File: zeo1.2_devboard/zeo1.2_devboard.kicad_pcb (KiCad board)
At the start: 4 copper layers, 25.4 x 25.4 mm, 96 parts, among them J1 USB_C_Receptacle_USB2.0_14P, J2 JST-PH Battery, J4 Micro_SD, Q2 BC817, Q3 BC817, SW1 Boot, SW2 RESET, U1 AP2112K-3.3, U10 ESP32-S3, U11 LSM6DS3, U12 BMM150, U13 W3011, U2 MCP73871, U3 BME280, U5 USBLC6-2SC6, U6 CP2102N-QFN24, U7 W25Q128JVSIQ, U8 ANT3216LL00R2400A, U9 MAX-M10S-00B, Y1 40MHz

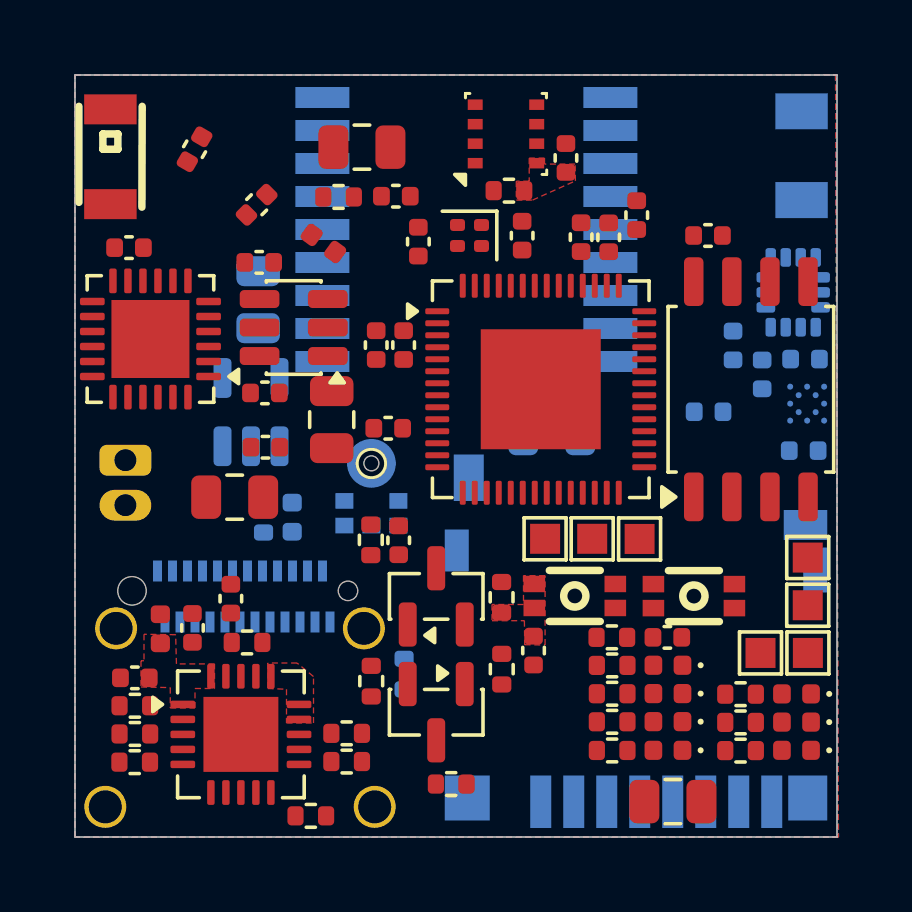
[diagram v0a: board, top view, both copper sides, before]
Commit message: new boards
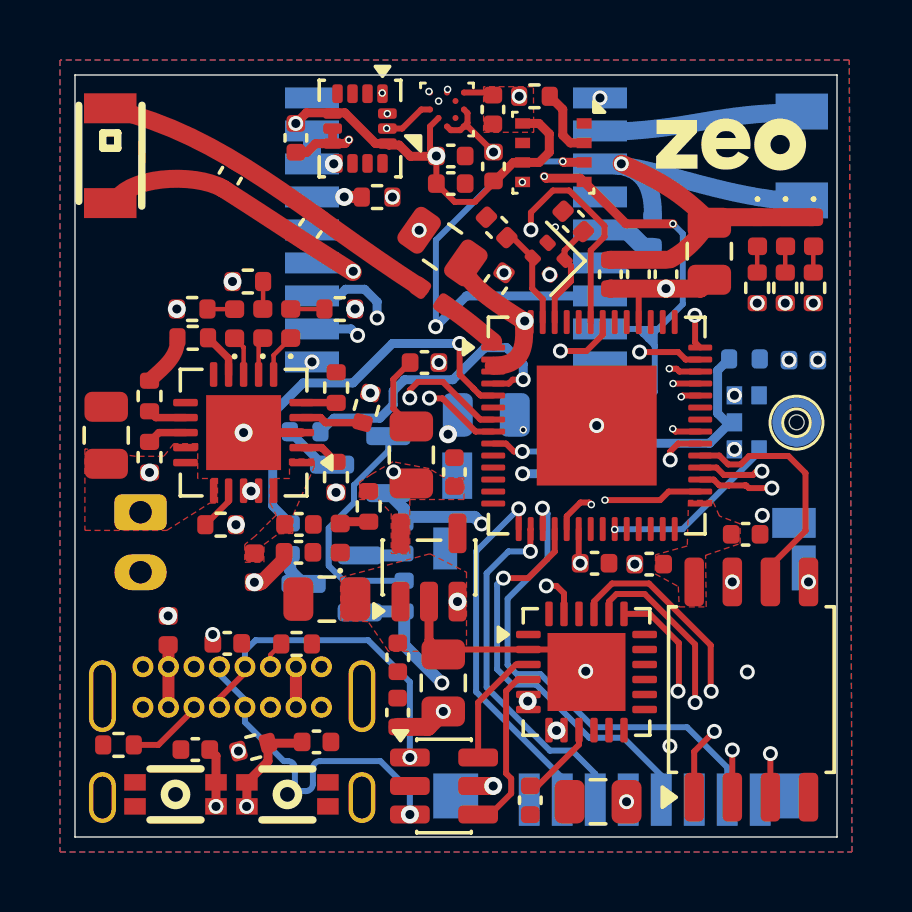
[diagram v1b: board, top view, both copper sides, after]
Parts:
- removed TP2, TP3, TP4, TP6, TP7, TP8, TP9: TestPoint, TestPoint:TestPoint_Pad_1.0x1.0mm
- added C11: 4.7uF, Capacitor_SMD:C_0805_2012Metric, F.Cu at (138.3, 99.3)
- added C12: 4.7uF, Capacitor_SMD:C_0805_2012Metric, B.Cu at (151.0, 98.6)
- added G***: LOGO, LOGO, F.Cu at (159.2, 89.6)
- C10, C38, Q2, Q3, R16, R22, R23, R24, R25: moved to B.Cu
- C19, C21, C26, C32, C33, C34, C9, F1, R1, R2, U1, U11, U12: moved to F.Cu
- J1: footprint Connector_USB:USB_C_Receptacle_Amphenol_12401610E4-2A_CircularHoles -> Connector_USB:USB_C_Receptacle_GCT_USB4085
- J2: footprint Connector_JST:JST_ZH_B2B-ZR_1x02_P1.50mm_Vertical -> Connector_JST:JST_PH_B2B-PH-K_1x02_P2.00mm_Vertical
- moved C17 22.8 mm to (152.5, 111.5), turned to 90 degrees
- moved R13 19.0 mm to (143.1, 94.2)
- moved D3 19.0 mm to (142.6, 95.6), turned to 90 degrees
- moved D2 19.0 mm to (144.5, 95.6), turned to 90 degrees
- moved R12 19.0 mm to (141.2, 95.1)
- moved D4 18.9 mm to (143.6, 95.6), turned to 90 degrees
- moved U6 18.3 mm to (154.3, 107.2), turned to 0 degrees
- moved C9 17.4 mm to (144.7, 89.4), turned to 90 degrees
- moved D5 17.3 mm to (161.9, 92.5), turned to -90 degrees
- moved R11 17.3 mm to (146.1, 95.1), turned to 180 degrees
- moved R7 16.4 mm to (141.2, 96.1), turned to 0 degrees
- moved D6 16.3 mm to (161.0, 92.5), turned to -90 degrees
- moved U5 16.1 mm to (149.6, 111.0), turned to 0 degrees
- moved C18 15.7 mm to (148.1, 108.5), turned to -90 degrees
- moved R20 15.6 mm to (161.9, 94.4), turned to 90 degrees
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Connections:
- C19 pad 2: unconnected-(C19-Pad2) -> +3V3
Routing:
- net /BOOT: track 0.00 -> 37.2 mm, vias 0 -> 2
- net /RX_TX: track 0.00 -> 33.3 mm, vias 0 -> 2
- net /EN: track 0.00 -> 33.2 mm, vias 0 -> 2
- net /SCL: track 0.00 -> 29.1 mm, vias 0 -> 4
- net /SDA: track 0.00 -> 28.8 mm, vias 0 -> 5
- net +3V3: track 0.00 -> 24.9 mm, vias 0 -> 17
- net /I2S_SD: track 0.00 -> 23.0 mm, vias 0 -> 2
- net /TX_RX: track 0.00 -> 22.4 mm, vias 0 -> 2
- net GND: track 0.00 -> 22.2 mm, vias 0 -> 23
- net /MCU/FLASH_CS: track 0.00 -> 18.9 mm, vias 0 -> 2
- net /GPS_RX: track 0.00 -> 18.6 mm, vias 0 -> 2
- net /GPS_TX: track 0.00 -> 18.0 mm, vias 0 -> 2
- net /MCU/~RTS: track 0.00 -> 17.1 mm, vias 0 -> 2
- net /MISO_DO: track 0.00 -> 16.4 mm, vias 0 -> 1
- net /MCU/FLASH_Q: track 0.00 -> 14.7 mm, vias 0 -> 2
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- added copper zone on In2.Cu, net +3V3
- added copper zone on F.Cu, net /+5V
- added copper zone on In2.Cu, net /+5V_USB
- added copper zone on F.Cu, net /MCU/VDD_SPI
- removed copper zone on F.Cu, net /BOOT
- removed copper zone on In2.Cu, net GND

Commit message: updated
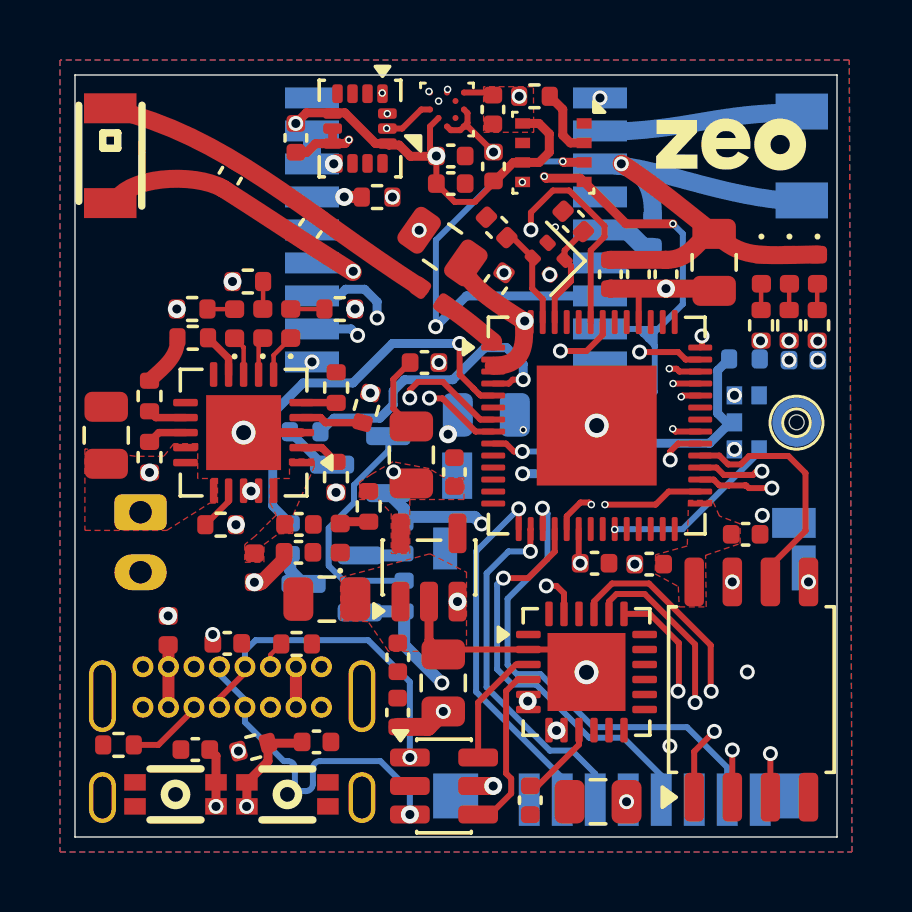
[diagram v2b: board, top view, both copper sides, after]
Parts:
- moved D5 1.26 mm to (162.1, 93.8)
- moved D6 1.26 mm to (161.1, 93.8)
- moved D7 1.26 mm to (160.2, 93.8)
- moved R20 1.26 mm to (162.0, 95.6)
- moved R21 1.26 mm to (161.1, 95.6)
- moved R26 1.26 mm to (160.2, 95.6)
- moved C37 0.40 mm to (158.6, 93.5)
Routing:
- net GND: track 22.2 -> 18.7 mm
- net /LED_R: track 6.35 -> 8.48 mm

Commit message: 1.2 updates
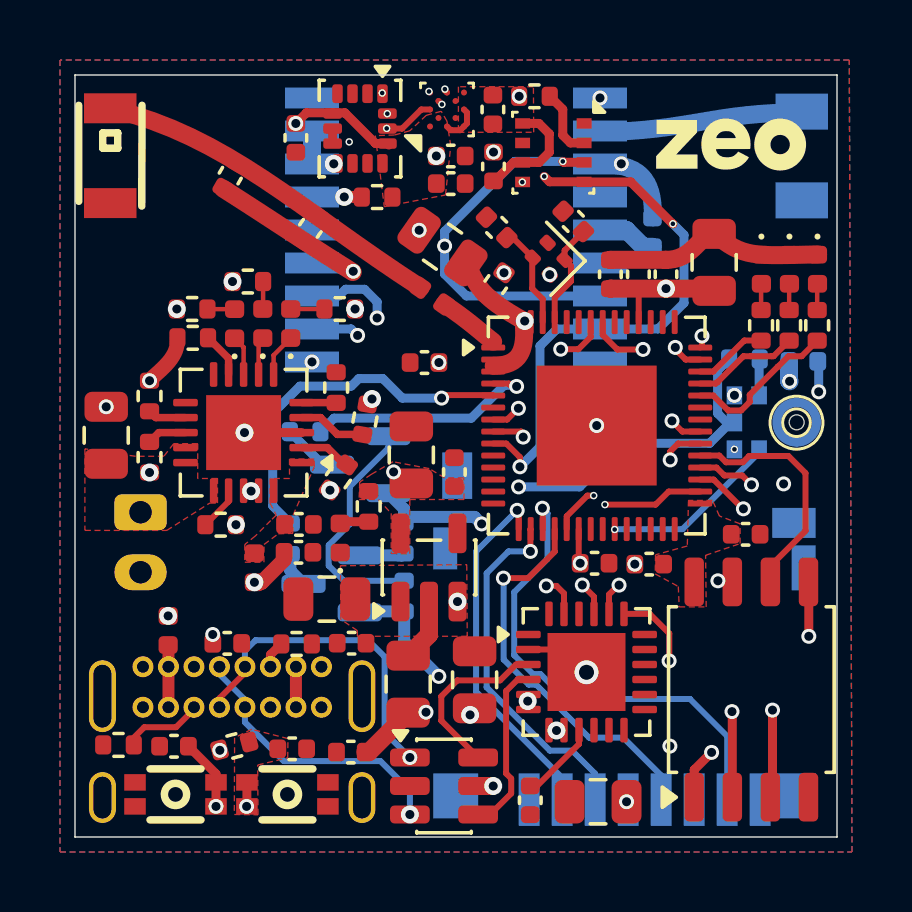
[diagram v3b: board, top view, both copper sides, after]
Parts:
- C12: moved to F.Cu
- moved C12 8.84 mm to (150.6, 107.5), turned to -90 degrees
- moved C18 2.04 mm to (146.5, 109.9), turned to 0 degrees
- moved C2 1.61 mm to (146.5, 106.2), turned to 0 degrees
- moved C19 1.17 mm to (148.4, 107.6)
- moved C14 0.84 mm to (144.5, 109.8)
- moved C13 0.72 mm to (140.6, 109.7)
- moved R19 0.63 mm to (142.6, 109.7)
- moved R4 0.39 mm to (147.0, 98.8), turned to -100 degrees
- moved R9 0.08 mm to (146.1, 100.7), turned to 55 degrees
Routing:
- net /RX_TX: track 33.3 -> 11.4 mm
- net /I2S_SD: track 23.0 -> 14.8 mm
- net /TX_RX: track 22.5 -> 15.5 mm
- net +3V3: track 25.0 -> 18.1 mm, vias 17 -> 16
- net /MCU/FLASH_D: track 9.83 -> 15.2 mm
- net /MCU/~RTS: track 17.1 -> 22.1 mm
- net /MCU/FLASH_HD: track 8.67 -> 13.5 mm
- net /EN: track 33.2 -> 28.9 mm
- net /BOOT: track 37.2 -> 33.0 mm
- net /LED_R: track 8.48 -> 5.21 mm, vias 2 -> 0
- net GND: track 18.7 -> 21.8 mm, vias 23 -> 22
- net /MCU/FLASH_CS: track 18.9 -> 16.5 mm
- net /+5V_USB: track 4.39 -> 6.63 mm
- net /SCL: track 29.1 -> 27.0 mm
- net /LED_B: track 4.49 -> 2.46 mm, vias 2 -> 0
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- added copper zone on F.Cu, net /EN
